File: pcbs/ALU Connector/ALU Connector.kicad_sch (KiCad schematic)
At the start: 54 parts, among them J101 Conn_02x20_Odd_Even, J102 Conn_02x20_Odd_Even, J103 Conn_01x04, J104 Conn_02x20_Odd_Even, J105 Conn_01x09, J106 Conn_01x06

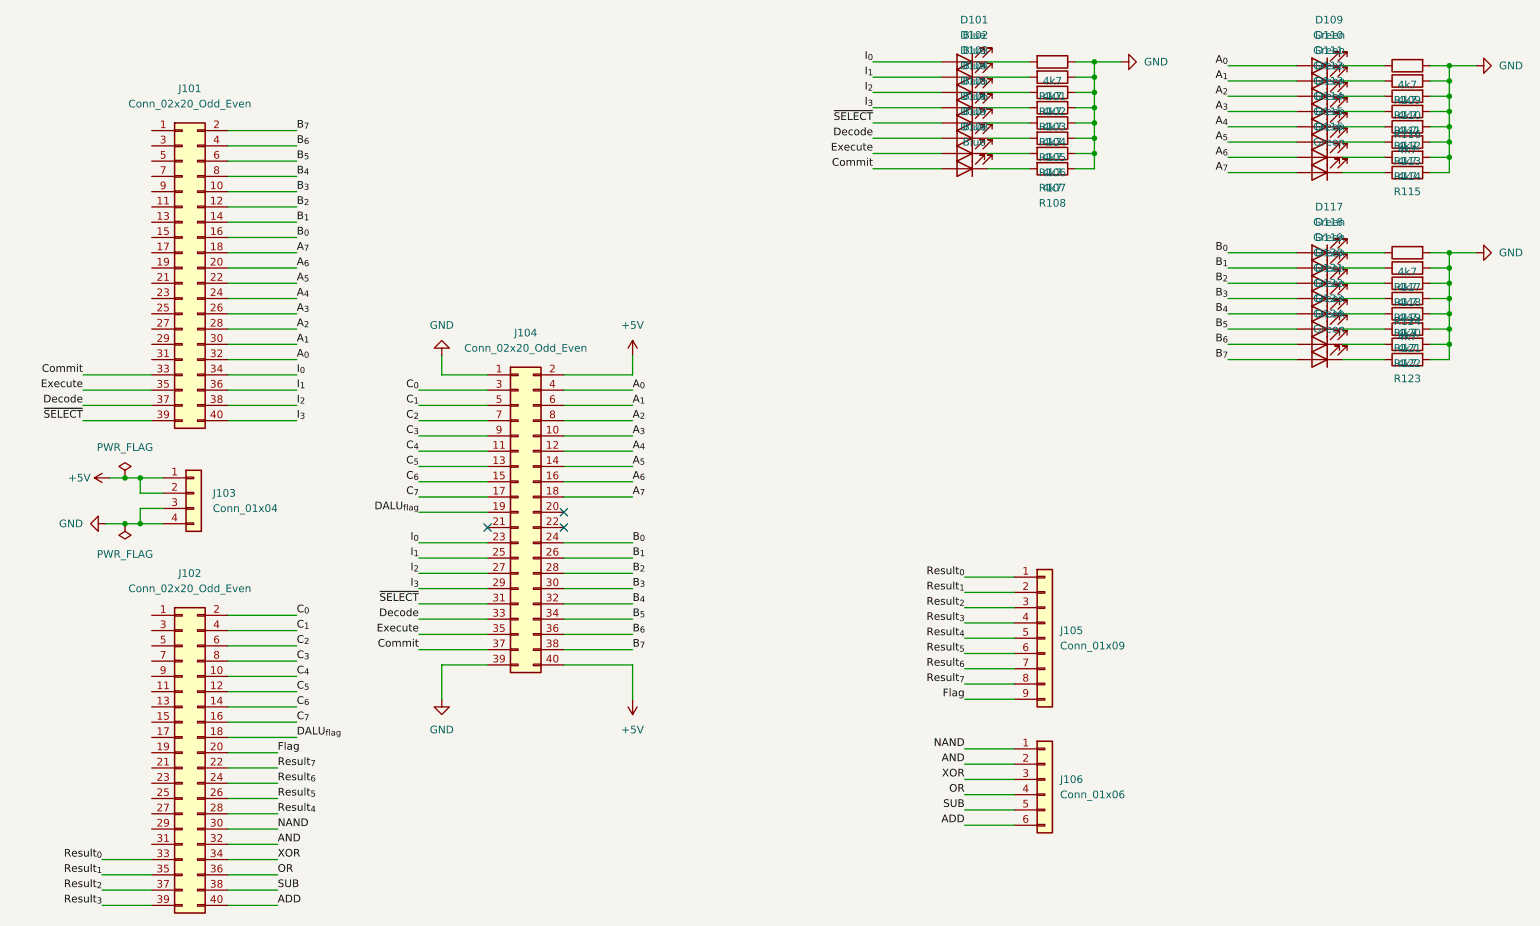
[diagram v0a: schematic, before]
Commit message: Realised a mistake
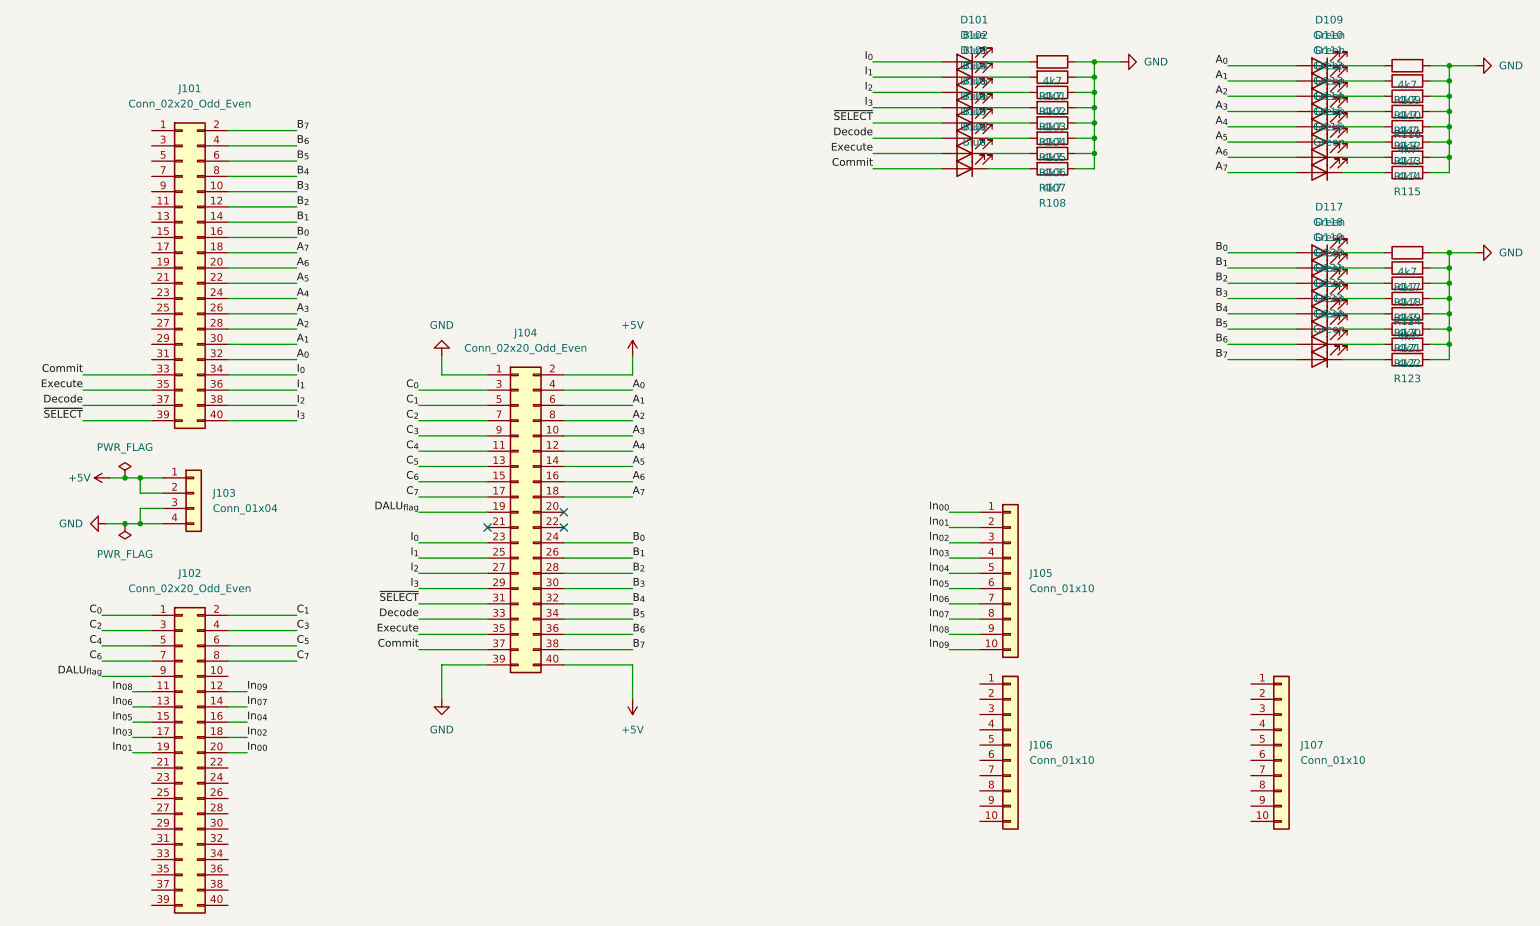
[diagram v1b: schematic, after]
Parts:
- removed J105: Conn_01x09, Connector_PinHeader_2.54mm:PinHeader_1x09_P2.54mm_Vertical, symbol Connector_Generic:Conn_01x09
- removed J106: Conn_01x06, Connector_PinHeader_2.54mm:PinHeader_1x06_P2.54mm_Vertical, symbol Connector_Generic:Conn_01x06
- added J105, J106, J107: Conn_01x10, Connector_PinHeader_2.54mm:PinHeader_1x10_P2.54mm_Vertical, symbol Connector_Generic:Conn_01x10
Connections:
- net C_{0}: now also J102.1 (Pin_1); no longer J102.2 (Pin_2)
- net C_{1}: now also J102.2 (Pin_2); no longer J102.4 (Pin_4)
- net C_{2}: now also J102.3 (Pin_3); no longer J102.6 (Pin_6)
- net C_{3}: now also J102.4 (Pin_4); no longer J102.8 (Pin_8)
- net C_{4}: now also J102.5 (Pin_5); no longer J102.10 (Pin_10)
- net C_{5}: now also J102.6 (Pin_6); no longer J102.12 (Pin_12)
- net C_{6}: now also J102.7 (Pin_7); no longer J102.14 (Pin_14)
- net C_{7}: now also J102.8 (Pin_8); no longer J102.16 (Pin_16)
- net DALU_{flag}: now also J102.9 (Pin_9); no longer J102.18 (Pin_18)
- net In_{08}: now reaches J102.11 (Pin_11)
- net In_{08}: now also J105.9 (Pin_9)
- net In_{06}: now reaches J102.13 (Pin_13)
- net In_{06}: now also J105.7 (Pin_7)
- net In_{05}: now reaches J102.15 (Pin_15)
- net In_{05}: now also J105.6 (Pin_6)
- net In_{03}: now reaches J102.17 (Pin_17)
- net In_{03}: now also J105.4 (Pin_4)
- net In_{01}: now reaches J102.19 (Pin_19)
- net In_{01}: now also J105.2 (Pin_2)
- net ADD: no longer names the net of J102.40 (Pin_40)
- net AND: no longer names the net of J102.32 (Pin_32)
- net Flag renamed In_{00}
- net In_{00}: now also J105.1 (Pin_1)
- net NAND: no longer names the net of J102.30 (Pin_30)
- net OR: no longer names the net of J102.36 (Pin_36)
- net Result_{0}: no longer names the net of J102.33 (Pin_33)
- net Result_{1}: no longer names the net of J102.35 (Pin_35)
- net Result_{2}: no longer names the net of J102.37 (Pin_37)
- net Result_{3}: no longer names the net of J102.39 (Pin_39)
- net Result_{4}: no longer names the net of J102.28 (Pin_28)
- net Result_{5}: no longer names the net of J102.26 (Pin_26)
- net Result_{6}: no longer names the net of J102.24 (Pin_24)
- net Result_{7}: no longer names the net of J102.22 (Pin_22)
- net SUB: no longer names the net of J102.38 (Pin_38)
- net XOR: no longer names the net of J102.34 (Pin_34)
- new net In_{02}: J102.18 (Pin_18), J105.3 (Pin_3)
- new net In_{04}: J102.16 (Pin_16), J105.5 (Pin_5)
- new net In_{07}: J102.14 (Pin_14), J105.8 (Pin_8)
- new net In_{09}: J102.12 (Pin_12), J105.10 (Pin_10)
